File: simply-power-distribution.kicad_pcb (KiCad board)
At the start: 2 copper layers, 33 x 25.4 mm, 9 parts, among them J1 55-21 Barrel Jack, J2 Power distribution, SW1 Power Switch

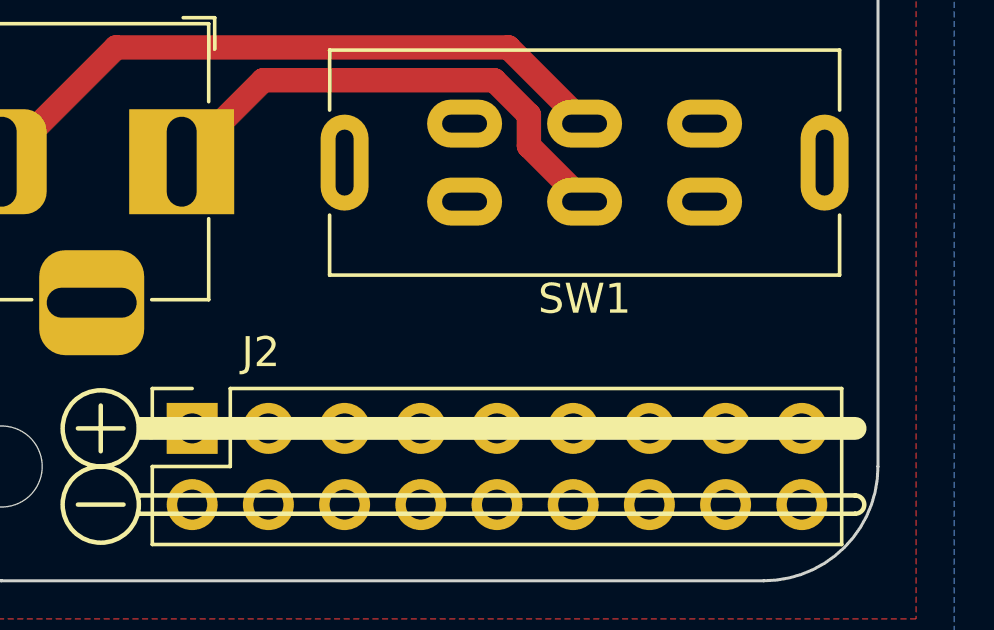
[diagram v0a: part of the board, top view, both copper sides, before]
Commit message: Prepare RC1
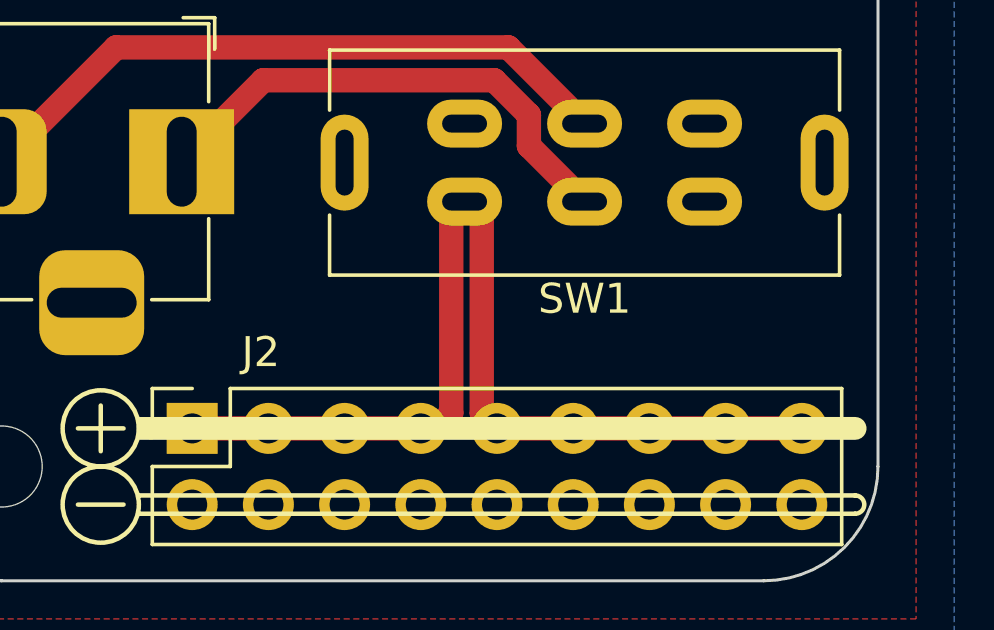
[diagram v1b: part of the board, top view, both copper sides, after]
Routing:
- net /VCC: track 0.00 -> 34.2 mm
- added copper zone on F.Cu, net /GND
- removed copper zone on F.Cu, net /VCC
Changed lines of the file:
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@@
   (title_block
     (title "Simply power distribution")
-    (date "2023-12-20")
-    (rev "v0.0.1-DRAFT")
+    (date "2024-01-21")
+    (rev "v0.0.1-RC1")
     (company "Sporniket")
     (comment 4 "Original repository : https://github.com/sporniket/simply-power-distribution")
@@
   (gr_arc (start 79.502 28.194) (mid 82.85762 29.21) (end 79.502 30.226)
     (stroke (width 0.15) (type default)) (layer "B.SilkS"))
-  (gr_rect (start 72.2872 46.0248) (end 71.8808 45.4152)
+  (gr_rect (start 71.8808 45.4152) (end 72.2872 46.0248)
     (stroke (width 0.15) (type solid)) (fill solid) (layer "B.SilkS"))
   (gr_line (start 86.106 29.21) (end 84.582 29.21)
@@
   (segment (start 84.2 33.02) (end 71.12 33.02) (width 0.8128) (layer "F.Cu") (net 2))
   (segment (start 86.74 35.56) (end 84.2 33.02) (width 0.8128) (layer "F.Cu") (net 2))
-  (zone (net 6) (net_name "/VCC") (layer "F.Cu") (hatch edge 0.5)
+  (segment (start 82.296 38.604) (end 82.74 38.16) (width 0.8128) (layer "F.Cu") (net 6))
+  (segment (start 81.788 45.72) (end 82.296 45.212) (width 0.8128) (layer "F.Cu") (net 6))
+  (segment (start 82.296 45.212) (end 82.296 38.604) (width 0.8128) (layer "F.Cu") (net 6))
+  (segment (start 93.98 45.72) (end 83.82 45.72) (width 0.8128) (layer "F.Cu") (net 6))
+  (segment (start 82.74 38.16) (end 83.312 38.732) (width 0.8128) (layer "F.Cu") (net 6))
+  (segment (start 83.312 38.732) (end 83.312 45.212) (width 0.8128) (layer "F.Cu") (net 6))
+  (segment (start 83.312 45.212) (end 83.82 45.72) (width 0.8128) (layer "F.Cu") (net 6))
+  (segment (start 73.66 45.72) (end 81.28 45.72) (width 0.8128) (layer "F.Cu") (net 6))
+  (segment (start 81.28 45.72) (end 81.788 45.72) (width 0.8128) (layer "F.Cu") (net 6))
+  (zone (net 5) (net_name "/GND") (layer "F.Cu") (hatch edge 0.5)
     (connect_pads (clearance 0.5))
     (min_thickness 0.25) (filled_areas_thickness no)
